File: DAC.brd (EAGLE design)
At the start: 99.1 x 55.9 mm, 76 parts, among them IC1 LM2662, IC2 PCM1793, IC3 OPA2134PA, J1 USBSMD, J2 RCJ-21XXMILL, U1 LDO-TPS78233, U2 PCM2707, Y1 12MHz/20pF

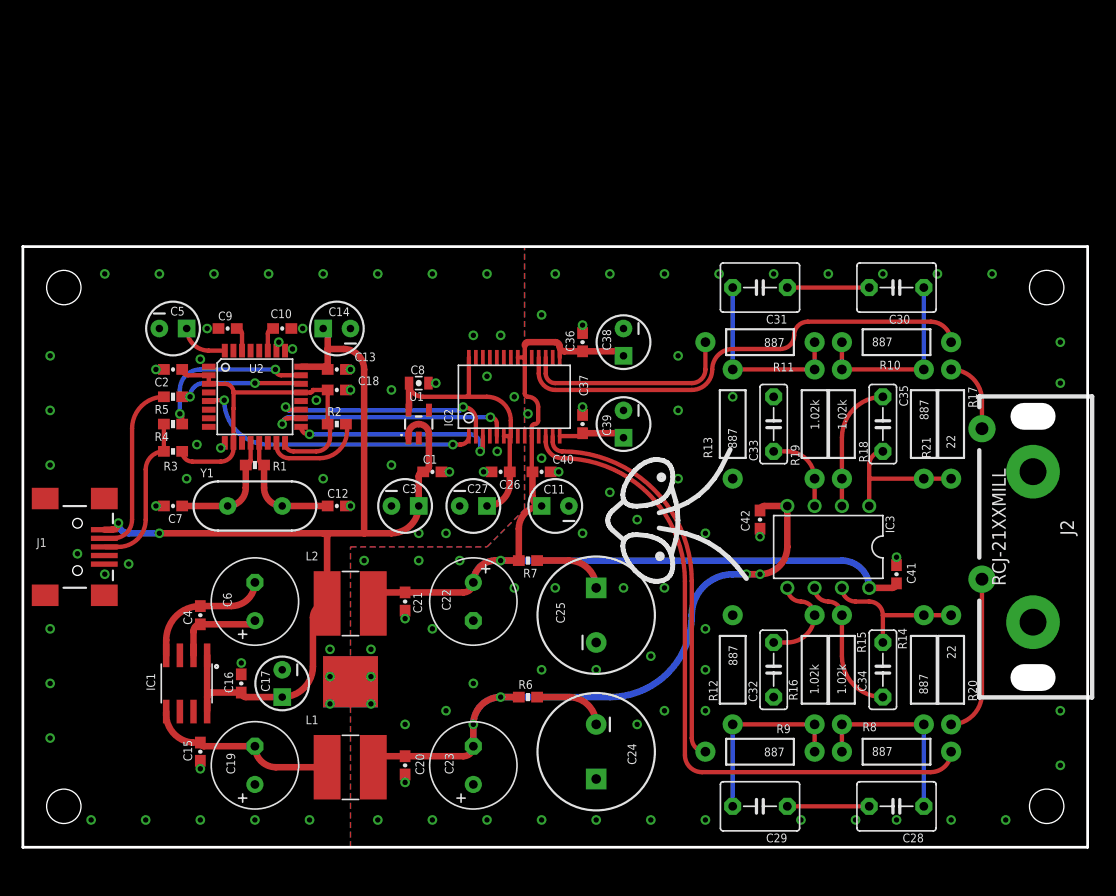
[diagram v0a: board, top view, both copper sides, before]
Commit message: Phone out
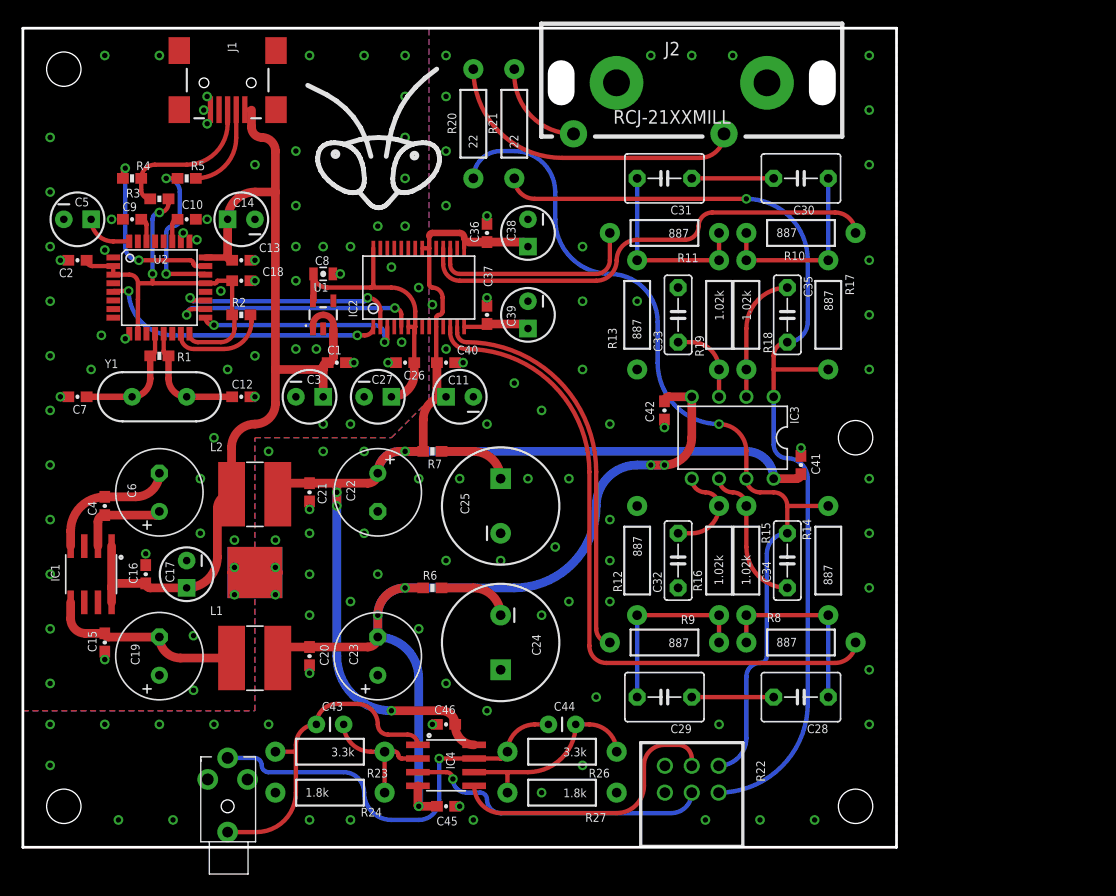
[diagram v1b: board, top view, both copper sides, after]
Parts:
- added C43, C44: 100pF, SparkFun-Capacitors:CAP-PTH-SMALL
- added C45, C46: 1.0uF, SparkFun-Capacitors:0603-CAP
- added IC4: LMH6643, my:SO08
- added J3: (no value), SparkFun-Connectors:STEREOJACK2.5MM_STEREOJACK2.5MM
- added R22: TD90, my:PTD902
- added R23, R26: 3.3k, SparkFun-Resistors:AXIAL-0.4
- added R24, R27: 1.8k, SparkFun-Resistors:AXIAL-0.4
- moved R20 67.5 mm to (41.9, 67.3), turned to 90 degrees
- moved J2 53.6 mm to (62.2, 71.1), turned to 0 degrees
- moved R21 49.3 mm to (45.7, 67.3)
- moved J1 45.4 mm to (19.1, 71.1), turned to 270 degrees
- moved LOGO1 45.2 mm to (33.0, 66.0), turned to 0 degrees
- moved R3 23.5 mm to (12.7, 60.3)
- moved R4 23.2 mm to (10.2, 62.2), turned to 0 degrees
- moved R5 20.4 mm to (15.2, 62.2), turned to 0 degrees
- moved R13 13.5 mm to (57.1, 49.5)
- moved R12 13.5 mm to (57.1, 26.7)
- moved C1 13.5 mm to (29.2, 45.1)
- moved C14 13.5 mm to (20.3, 58.4)
- moved C21 13.5 mm to (26.7, 33.0)
- moved C26 13.5 mm to (35.6, 45.1)
- moved C35 13.5 mm to (71.1, 49.5)
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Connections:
- net N$6 renamed D+*
- net N$7 renamed D-*
- removed net N$100: C35.2, IC3.1, R17.P$2, R21.P$1
- removed net N$101: C34.2, IC3.7, R14.P$2, R20.P$1
- new net HP_L: C43.1, IC4.1, J3.SHIELD, R23.P$2
- new net HP_R: C44.1, IC4.7, J3.TIP, R26.P$2
- new net N$12: IC4.3, R22.R1.2
- new net N$14: C43.2, IC4.2, R23.P$1, R24.P$2
- new net N$15: IC4.5, R22.R2.2
- new net N$19: C44.2, IC4.6, R26.P$1, R27.P$2
- new net OUT_L*: C35.2, IC3.1, R17.P$2, R21.P$1, R22.R1.3
- new net OUT_R*: C34.2, IC3.7, R14.P$2, R20.P$1, R22.R2.3
- net +5V: now also C46.1, IC4.8
- net -5V: now also C45.1, IC4.4
- net AGND: now also C45.2, C46.2, J3.RING1, R22.R1.1, R22.R2.1, R24.P$1, R27.P$1
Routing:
- net OUT_L*: track 0.00 -> 91.1 mm, vias 0 -> 1
- net OUT_R*: track 0.00 -> 79.8 mm, vias 0 -> 1
- net HP_R: track 0.00 -> 38.1 mm, vias 0 -> 1
- net +5V: track 90.2 -> 123.8 mm, vias 1 -> 4
- net HP_L: track 0.00 -> 28.7 mm
- net N$12: track 0.00 -> 27.8 mm, vias 0 -> 1
- net N$15: track 0.00 -> 26.2 mm
- net -5V: track 63.3 -> 84.3 mm, vias 4 -> 5
- net N$19: track 0.00 -> 18.1 mm
- net N$101: track 13.8 -> 0.00 mm
- net N$100: track 13.2 -> 0.00 mm
- net OUT_R: track 14.7 -> 27.7 mm
- net N$14: track 0.00 -> 12.0 mm
- net VCC: track 96.7 -> 88.6 mm, vias 2 -> 0
- net D-: track 16.0 -> 7.95 mm
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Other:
- board size 99.1 x 55.9 mm -> 81.3 x 76.2 mm
